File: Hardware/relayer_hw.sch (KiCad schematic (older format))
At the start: 48 parts

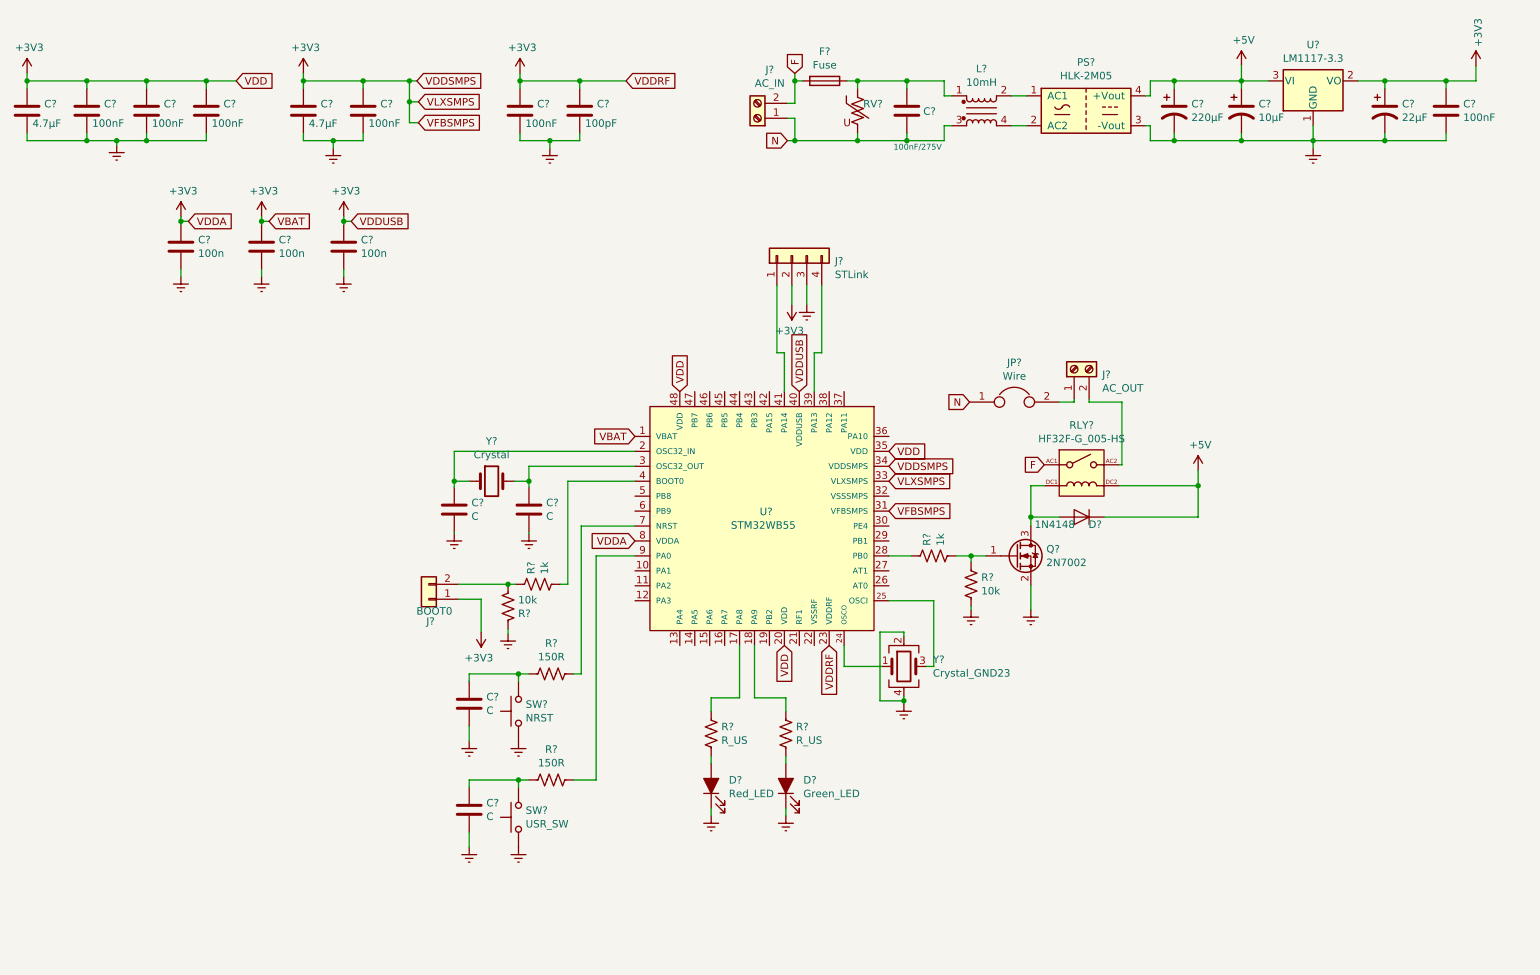
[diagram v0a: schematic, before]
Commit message: Circuito RF/ Reorganização prática do hardware
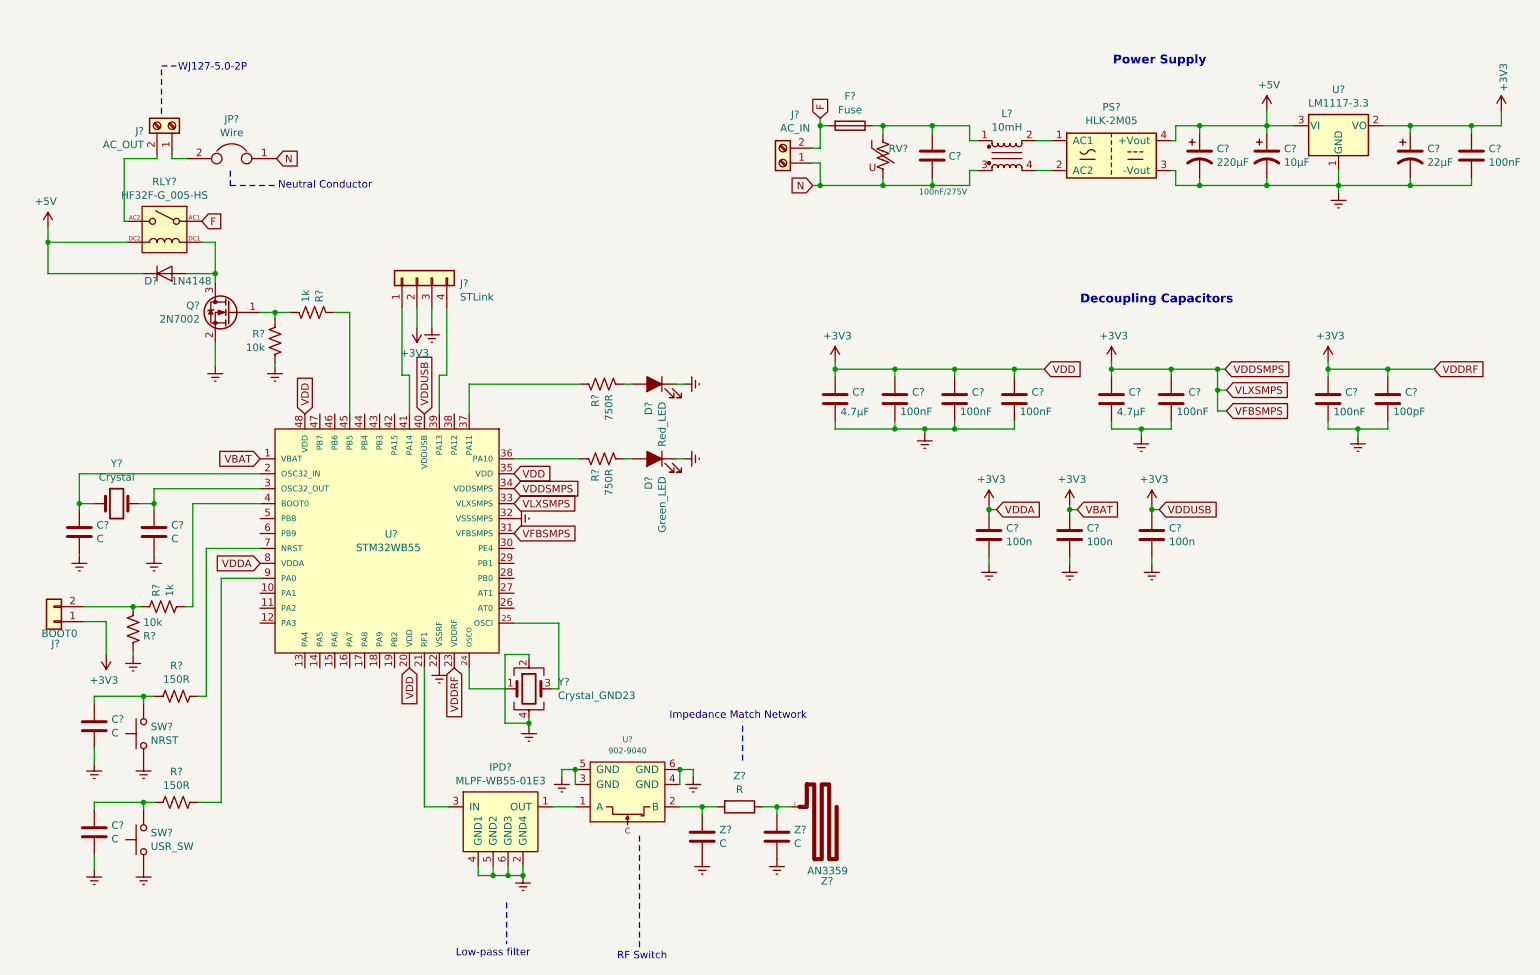
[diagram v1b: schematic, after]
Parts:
- added IPD?: MLPF-WB55-01E3, symbol Usr_Sym:MLPF-WB55-01E3
- added U?: 902-9040, symbol Usr_Sym:902-9040-fermbuddy
- added Z?: AN3359, symbol Usr_Sym:AN3359
- added Z?: R, symbol Device:R
- added Z? (x2): C, symbol Device:C
- C?: footprint (none) -> Capacitor_THT:C_Rect_L18.0mm_W6.0mm_P15.00mm_FKS3_FKP3
- J?: footprint (none) -> TerminalBlock:TerminalBlock_bornier-2_P5.08mm
- R? (x2): value R_US -> 750R
- RV?: footprint (none) -> Varistor:RV_Disc_D12mm_W6.1mm_P7.5mm
- U?: footprint (none) -> Package_TO_SOT_SMD:SOT-223
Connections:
- net at R?.1: now also U?.45 (PB5); no longer U?.28 (PB0)
- net at U?.17 (PA8): no longer R?.1
- net at U?.18 (PA9): no longer R?.1
- net at U?.21 (RF1): now also IPD?.3 (IN)
- net at U?.36 (PA10): now also R?.1
- net at U?.37 (PA11): now also R?.1
- new net: IPD?.1 (OUT), U?.1 (A)
- new net: U?.2 (B), Z?.1, Z?.2
- new net: U?.3 (GND), U?.5 (GND)
- new net: U?.4 (GND), U?.6 (GND)
- new net: Z?.1, Z?.1, Z?.1 (RF)
- new net: IPD?.2 (GND4), IPD?.4 (GND1), IPD?.5 (GND2), IPD?.6 (GND3)
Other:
- note added: "Decoupling Capacitors"
- note added: "Impedance Match Network"
- note added: "Low-pass filter\n"
- note added: "Neutral Conductor"
- note added: "Power Supply"
- note added: "RF Switch"
- note added: "WJ127-5.0-2P"
- moved on the sheet: C?, D?, F?, J?, JP?, L?, PS?, Q?, R?, RLY?, RV?, SW?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
